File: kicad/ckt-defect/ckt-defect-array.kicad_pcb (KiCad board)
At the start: 2 copper layers, 114.3 x 188 mm, 316 parts, among them J1 Screw_Terminal_01x02, J10 Micro_SD_Card_Det_Hirose_DM3AT, J11 690-005-299-043, J12 SM04B-SRSS, J13 Conn_01x03, J14 Conn_01x03, J2 SM04B-SRSS, J3 SM04B-SRSS, J4 SM04B-SRSS, J5 SM04B-SRSS, J6 SM04B-SRSS, J7 SM04B-SRSS, J8 SM04B-SRSS, J9 Screw_Terminal_01x02, SW5 FSM4JSMA, SW6 FSM4JSMA, U1 MAX98357AETE+T, U2 AP63205WU, U3 TMP1075D, U4 AZ1117-3.3, U5 ESP32-S2-SOLO, U6 74LVC14, U7 TLP241A

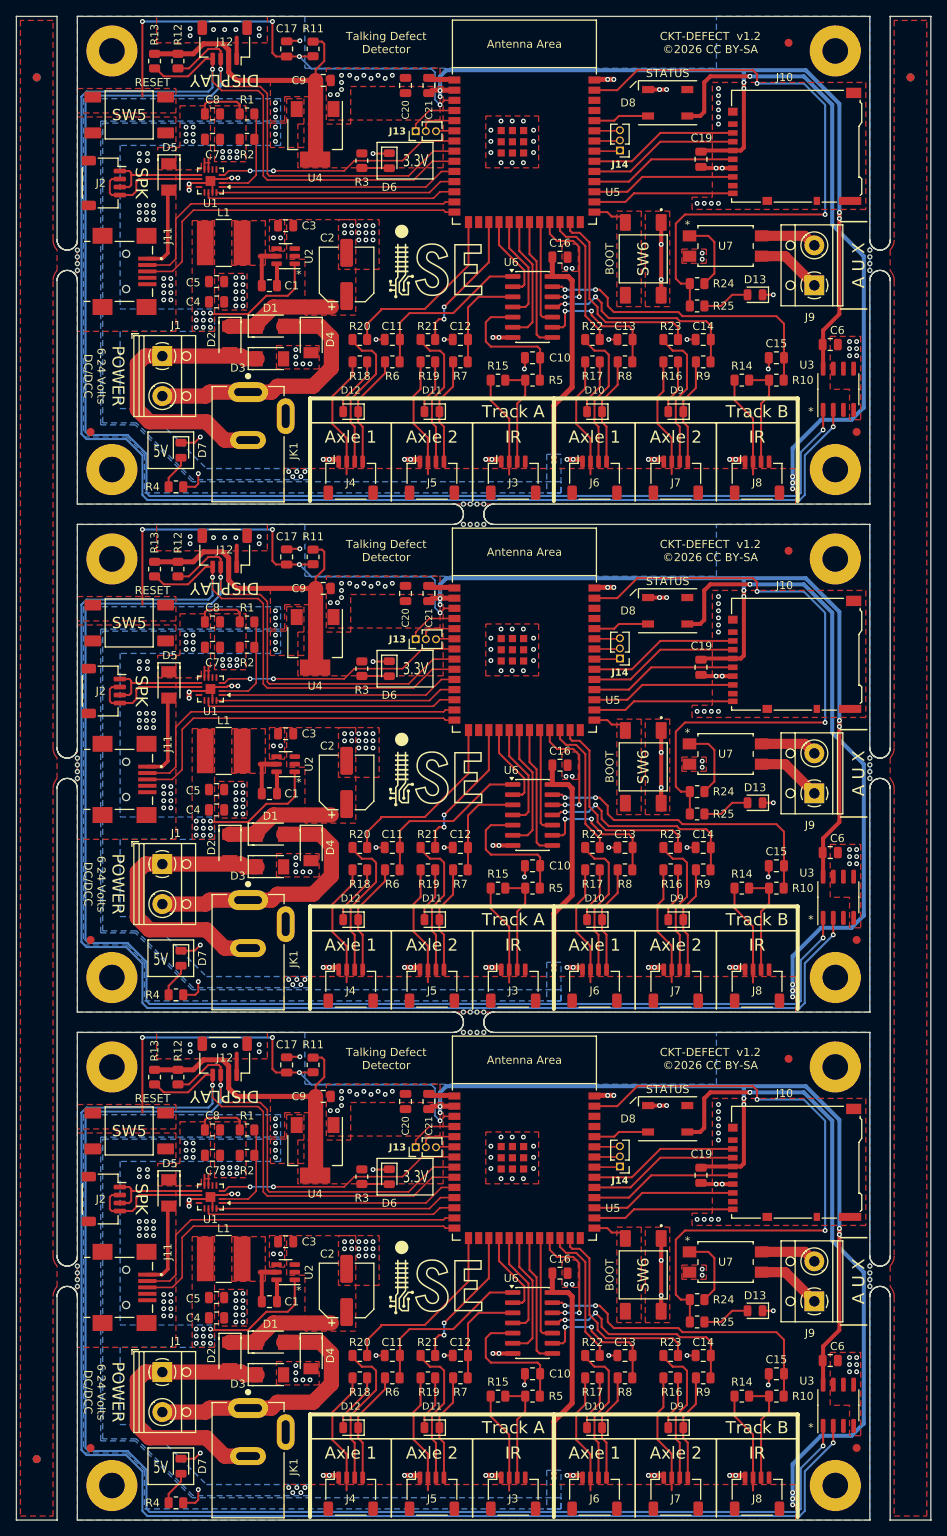
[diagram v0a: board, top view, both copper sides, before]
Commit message: New array
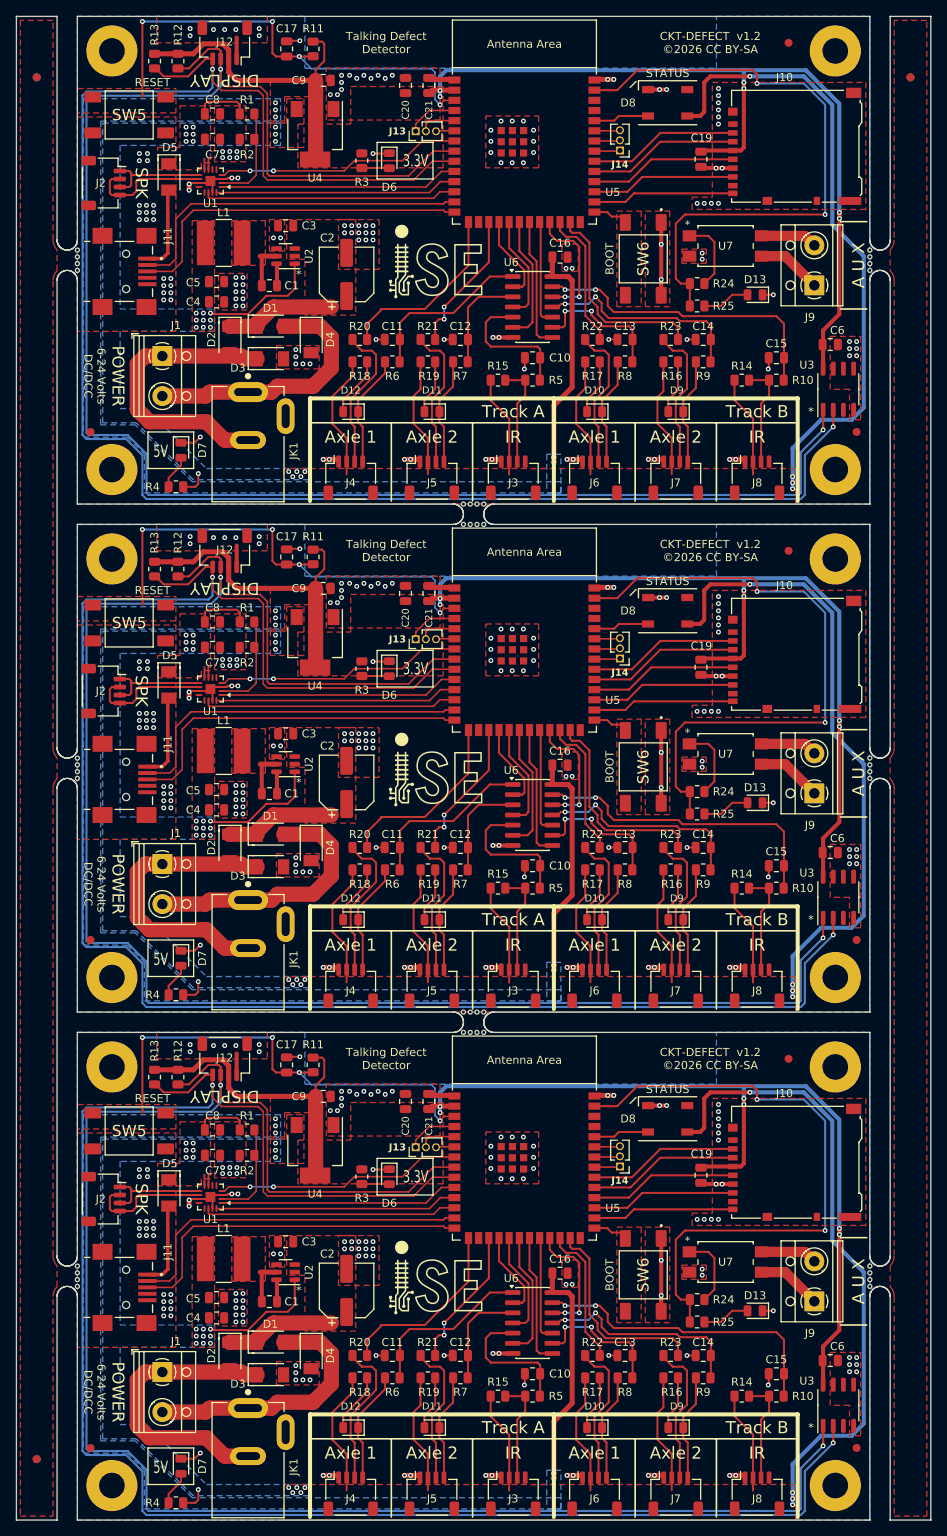
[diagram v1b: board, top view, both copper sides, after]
